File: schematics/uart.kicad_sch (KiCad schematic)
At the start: 8 parts, among them U10 W65C51NxP, U27 W65C22SxP, Y4 1.8432MHz

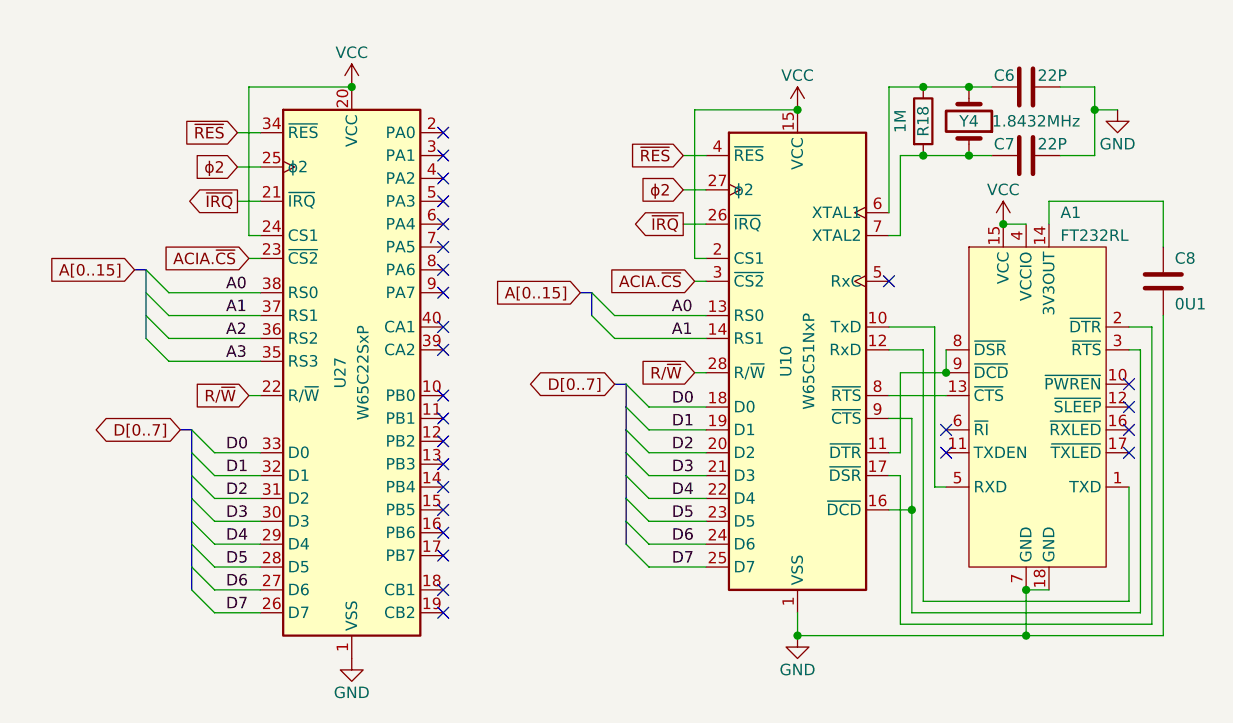
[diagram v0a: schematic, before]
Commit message: added phi0 for write latch timing
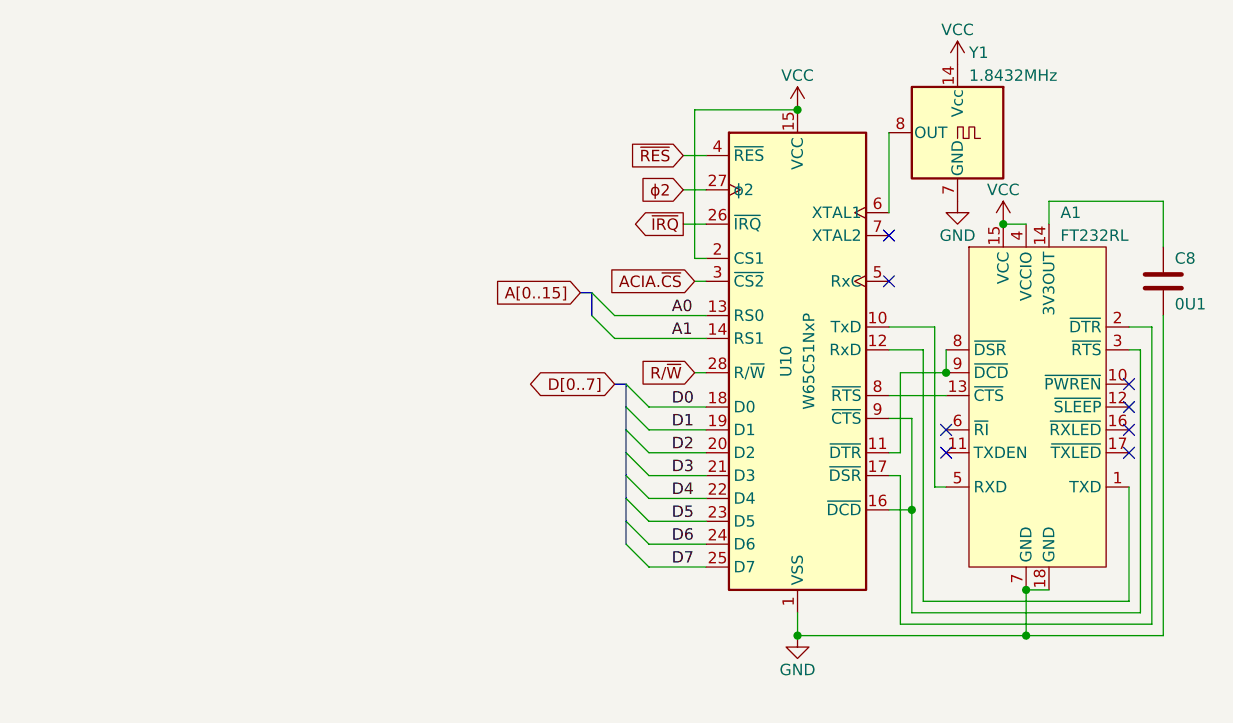
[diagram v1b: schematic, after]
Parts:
- removed C6, C7: 22P, symbol Device:C
- removed R18: 1M, symbol Device:R
- removed U27: W65C22SxP, Package_DIP:DIP-40_W15.24mm, symbol 65xx-library:W65C22SxP
- removed Y4: 1.8432MHz, symbol Device:Crystal
- added Y1: 1.8432MHz, Oscillator:Oscillator_DIP-14, symbol Oscillator:ACO-xxxMHz
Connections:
- net GND: now also Y1.7 (GND)
- net VCC: now also Y1.14 (Vcc)
- net at U10.6 (XTAL1): now also Y1.8 (OUT)
- no-connect marks 27 -> 8
